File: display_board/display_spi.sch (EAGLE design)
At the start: 18 parts

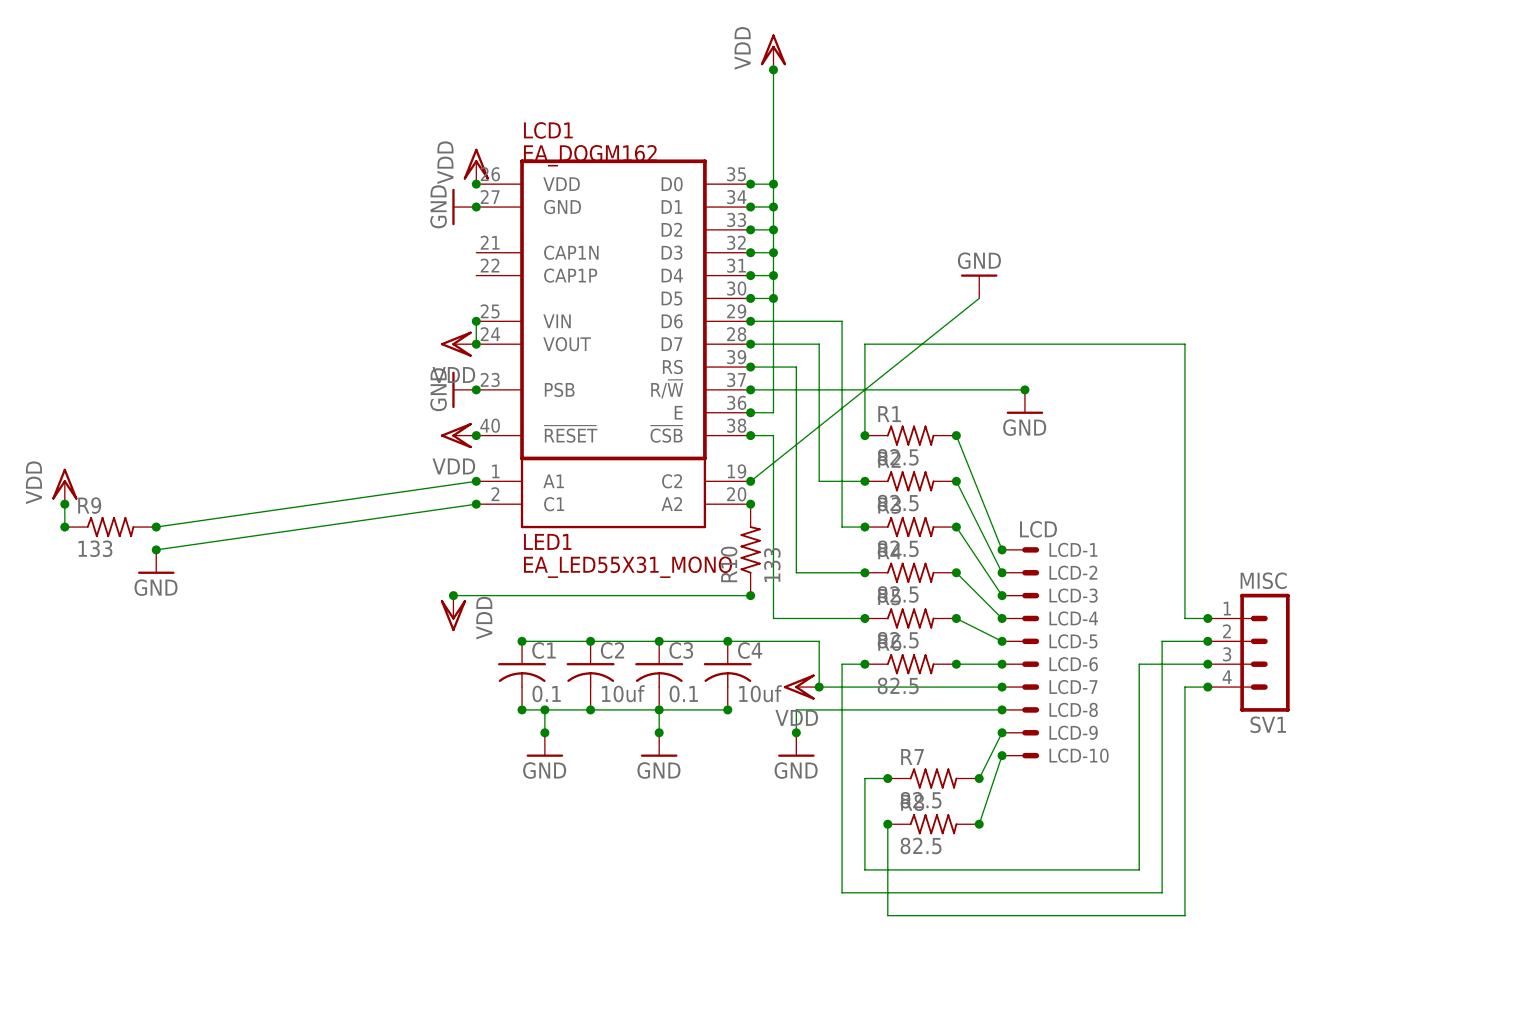
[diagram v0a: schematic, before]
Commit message: update
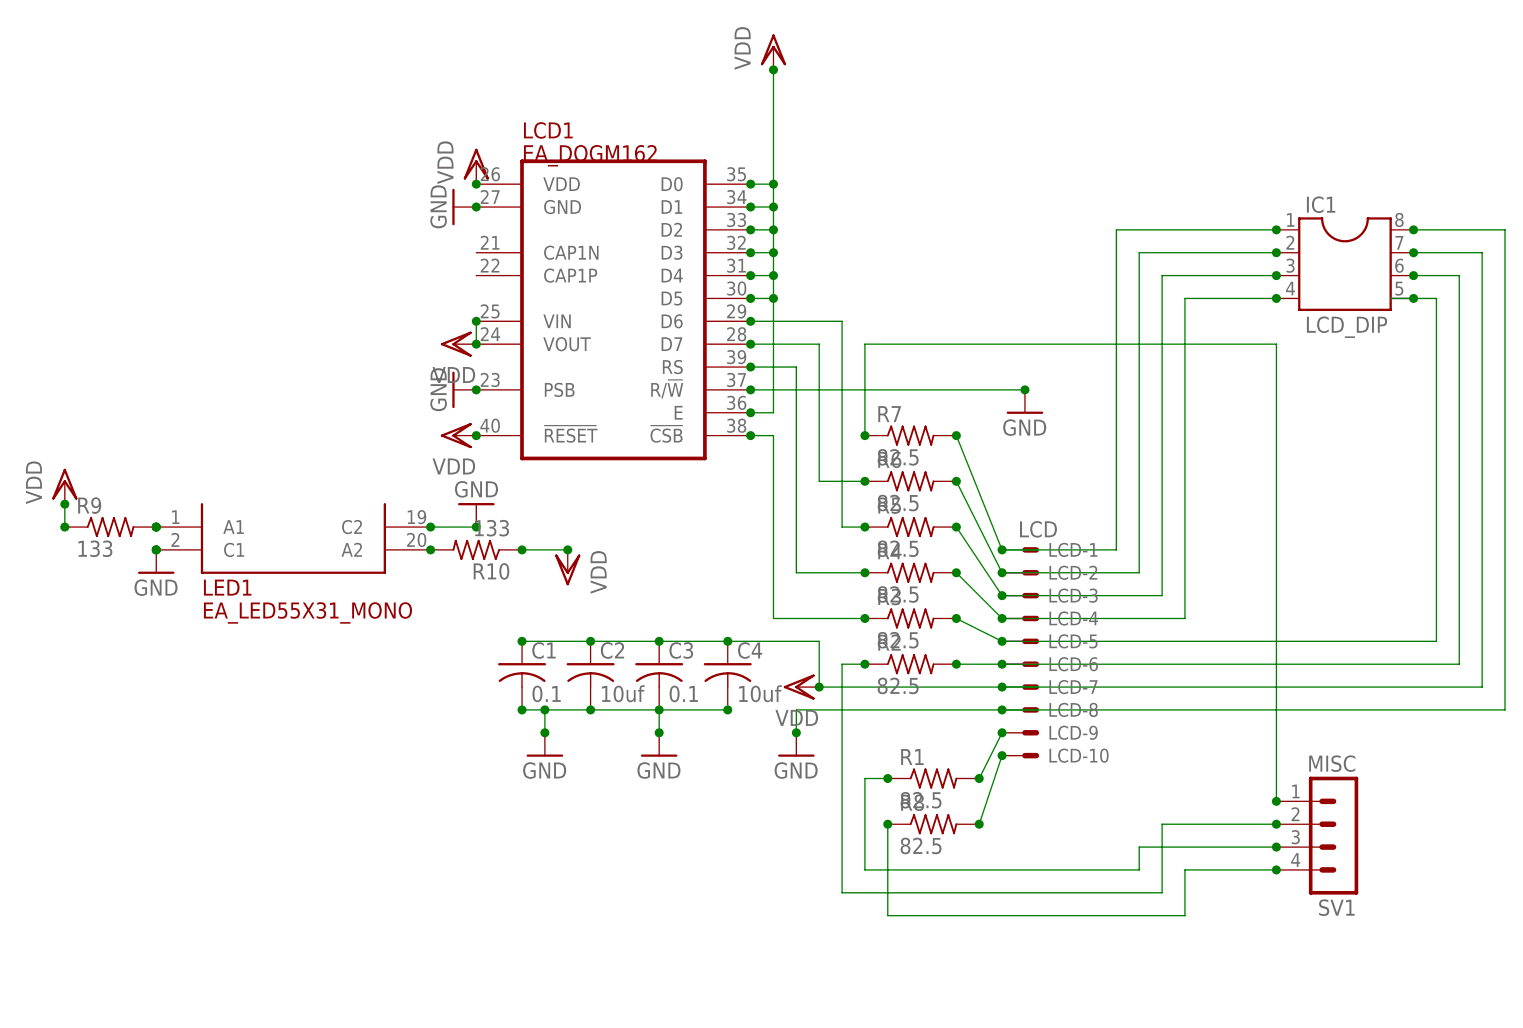
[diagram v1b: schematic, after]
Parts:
- added IC1: LCD_DIP, ic-package:DIL8S
- R1, R2, R3, R4, R5, R6, R7, R8: device rcl:R-US_R1206 -> rcl:R-US_R0805
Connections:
- net GND: now also IC1.8
- net N$1: now also IC1.1, R7.2; no longer R1.2
- net N$10: now also R5.1; no longer R3.1
- net N$12: now also R3.1; no longer R5.1
- net N$13: now also R7.1; no longer R1.1
- net N$14: now also R2.1; no longer R6.1
- net N$15: now also R1.1; no longer R7.1
- net N$2: now also IC1.2, R6.2; no longer R2.2
- net N$3: now also IC1.3, R5.2; no longer R3.2
- net N$4: now also IC1.4
- net N$5: now also IC1.5, R3.2; no longer R5.2
- net N$6: now also IC1.6, R2.2; no longer R6.2
- net N$7: now also R1.2; no longer R7.2
- net N$9: now also R6.1; no longer R2.1
- net VDD: now also IC1.7
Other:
- moved on the sheet: LED1, R1, R10, R2, R3, R5, R6, R7, SV1

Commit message: up mod display board
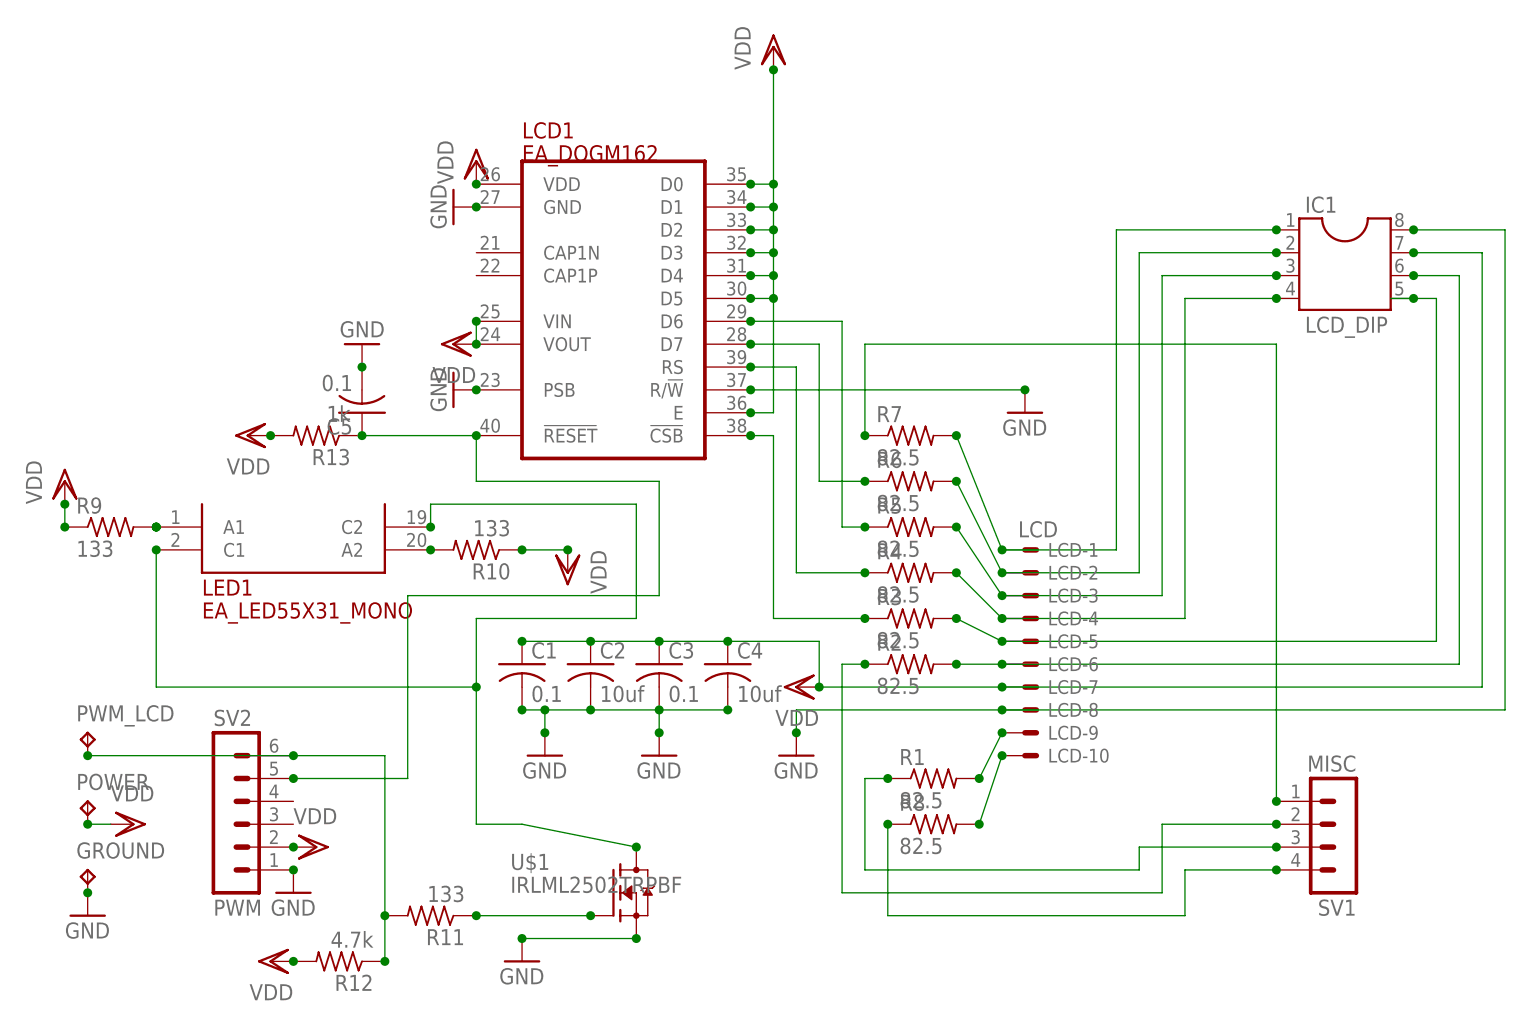
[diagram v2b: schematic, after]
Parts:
- added C5: 0.1, rcl:C-USC1206
- added GROUND, POWER: TPB1,27, testpad:TPB1,27
- added PWM_LCD: PWM, testpad:TPB1,27
- added R11: 133, rcl:R-US_R1206
- added R12: 4.7k, rcl:R-US_R1206
- added R13: 1k, rcl:R-US_R1206
- added SV2: PWM, con-lstb:MA06-1
- added U$1: IRLML2502TRPBF, IRLML2502TRPBF:IRLML2502TRPBF
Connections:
- new net N$19: LED1.C1, LED1.C2, U$1.D
- new net N$20: C5.1, LCD1.!RESET!, R13.1, SV2.5
- new net N$21: R11.1, U$1.G
- new net N$22: PWM_LCD.TP, R11.2, R12.1, SV2.6
- net GND: now also C5.2, GROUND.TP, SV2.1, U$1.S; no longer LED1.C1, LED1.C2
- net VDD: now also POWER.TP, R12.2, R13.2, SV2.2; no longer LCD1.!RESET!
